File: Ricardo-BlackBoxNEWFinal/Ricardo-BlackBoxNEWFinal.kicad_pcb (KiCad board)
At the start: 4 copper layers, 44 x 50 mm, 87 parts, among them IC1 XTSD08GLGEAG, IC2 CP2102N-A02-GQFN24, J1 RBUS, J2 USB_C_Receptacle_USB2.0, U1 ESP32-S3, U2 SN65HVD230, U3 LM66200DRLR, U4 MAX77827AEFD+T, U5 SC4215, Y1 40MHz±10ppm

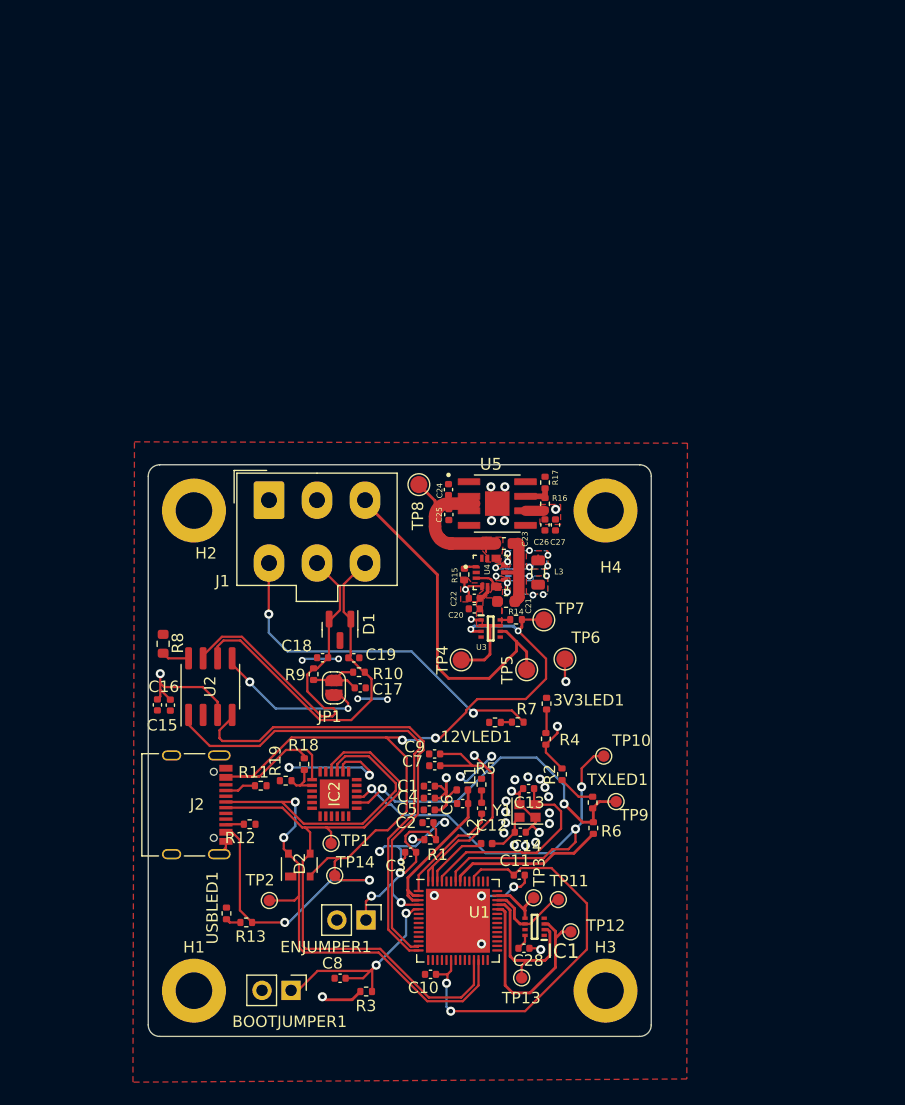
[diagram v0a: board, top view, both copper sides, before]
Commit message: Ricardo-BlackBoxFinal_15_08_2023
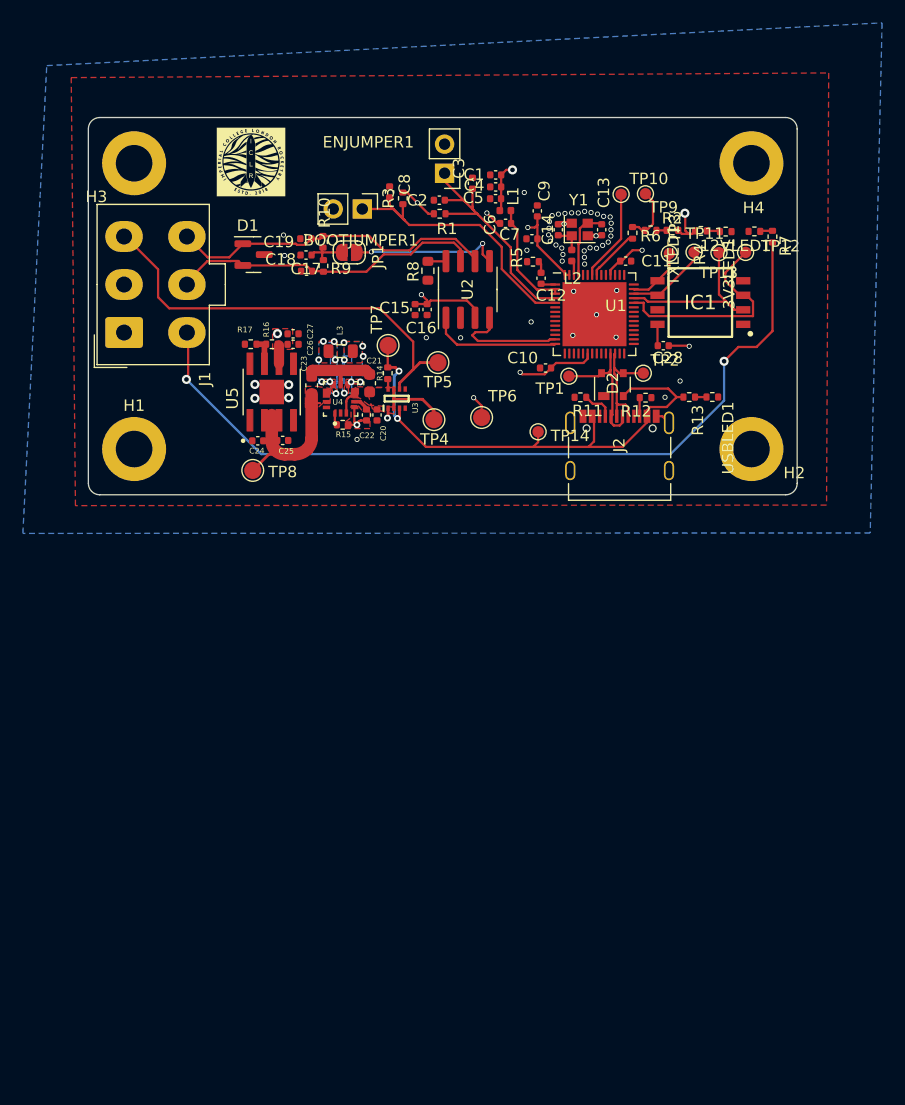
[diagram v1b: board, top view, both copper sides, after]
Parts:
- removed IC2: CP2102N-A02-GQFN24, iclr:QFN50P400X400X80-25N
- removed R18: 22.1k, Resistor_SMD:R_0402_1005Metric
- removed R19: 47.5k, Resistor_SMD:R_0402_1005Metric
- added G***: LOGO, LOGO, F.Cu at (128.7, 45.1)
- IC1: footprint iclr:SOTFL50P160X60-8N -> iclr:SON127P800X600X95-8N
- moved H3 83.3 mm to (118.5, 45.2)
- moved R3 69.5 mm to (142.0, 48.3), turned to -90 degrees
- moved C8 68.9 mm to (140.8, 47.7), turned to 90 degrees
- moved BOOTJUMPER1 68.6 mm to (138.4, 49.2)
- moved TP13 65.7 mm to (169.6, 53.0)
- moved ENJUMPER1 65.7 mm to (145.6, 46.1), turned to 180 degrees
- moved USBLED1 62.0 mm to (169.1, 65.7), turned to 180 degrees
- moved TP12 61.4 mm to (172.0, 53.0)
- moved R13 60.1 mm to (167.0, 65.7), turned to 0 degrees
- moved C3 58.8 mm to (148.1, 47.0), turned to 90 degrees
- moved TP11 57.9 mm to (167.4, 53.0)
- moved TP3 57.6 mm to (165.3, 53.1)
- moved TP2 56.5 mm to (163.0, 63.6)
- moved IC1 56.5 mm to (168.0, 57.4)
- moved R1 54.8 mm to (145.2, 49.6)
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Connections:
- D2 pad 3: /Data- -> /Data+
- D2 pad 4: /Data+ -> /Data-
- J2 pad B6: unconnected-(J2-D+-PadB6) -> /Data+
- J2 pad B7: unconnected-(J2-D--PadB7) -> /Data-
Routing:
- net VBUS: track 99.9 -> 46.6 mm, vias 6 -> 2
- net /Data+: track 62.6 -> 10.6 mm, vias 2 -> 0
- net +3V3: track 91.5 -> 42.7 mm, vias 11 -> 10
- net /Data-: track 58.0 -> 11.8 mm
- net +12V: track 31.8 -> 72.4 mm
- net /RXD: track 44.1 -> 8.09 mm, vias 3 -> 0
- net GND: track 62.0 -> 28.5 mm, vias 37 -> 52
- net /CAN_TX: track 43.7 -> 11.4 mm
- net /CAN_RX: track 42.0 -> 10.3 mm
- net /TXD: track 30.1 -> 5.06 mm, vias 2 -> 0
- net Net-(U1-XTAL_N): track 18.1 -> 6.24 mm
- net Net-(U1-U0TXD/PROG/GPIO43): track 13.6 -> 4.69 mm
- net Net-(U1-LNA_IN/RF): track 9.57 -> 1.26 mm
- net RBUS_uC_V: track 31.0 -> 37.6 mm
- net /CAN+: track 32.5 -> 27.7 mm
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- added copper zone on B.Cu, net GND
- removed copper zone on In2.Cu, net GND
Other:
- board size 44 x 50 mm -> 62 x 33 mm
